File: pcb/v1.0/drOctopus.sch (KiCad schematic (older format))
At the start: 47 parts, among them CON1 Servo, CON2 Servo, CON3 Heater, CON4 +12V, CON5 BEC, CON6 Motor, CON7 FAN1, CON8 FAN2, Q1 16MHz, SW1 RESET, T1 IRLR2905PBF, T2 IRLML6244TRPBF, T3 IRLML6244TRPBF, T4 IRLML6244TRPBF, U1 ATmega328-AU, U2 78M05CDT, U3 ESP-01, U4 AMS1117-3.3

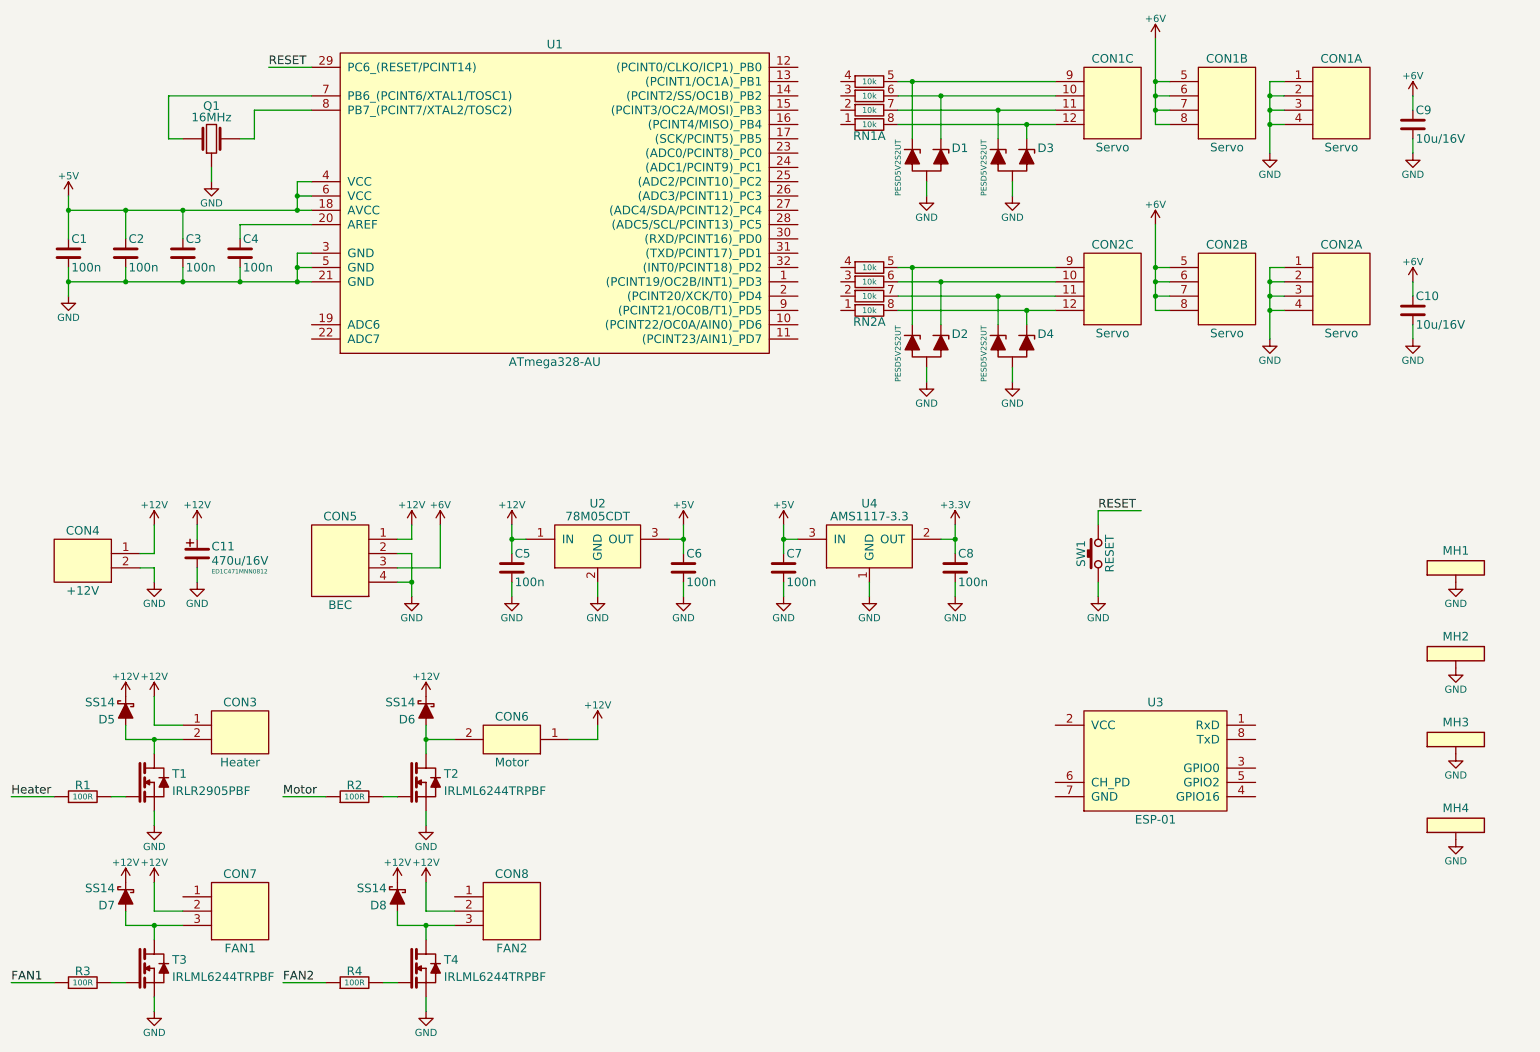
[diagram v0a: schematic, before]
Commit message: Working on new PCB
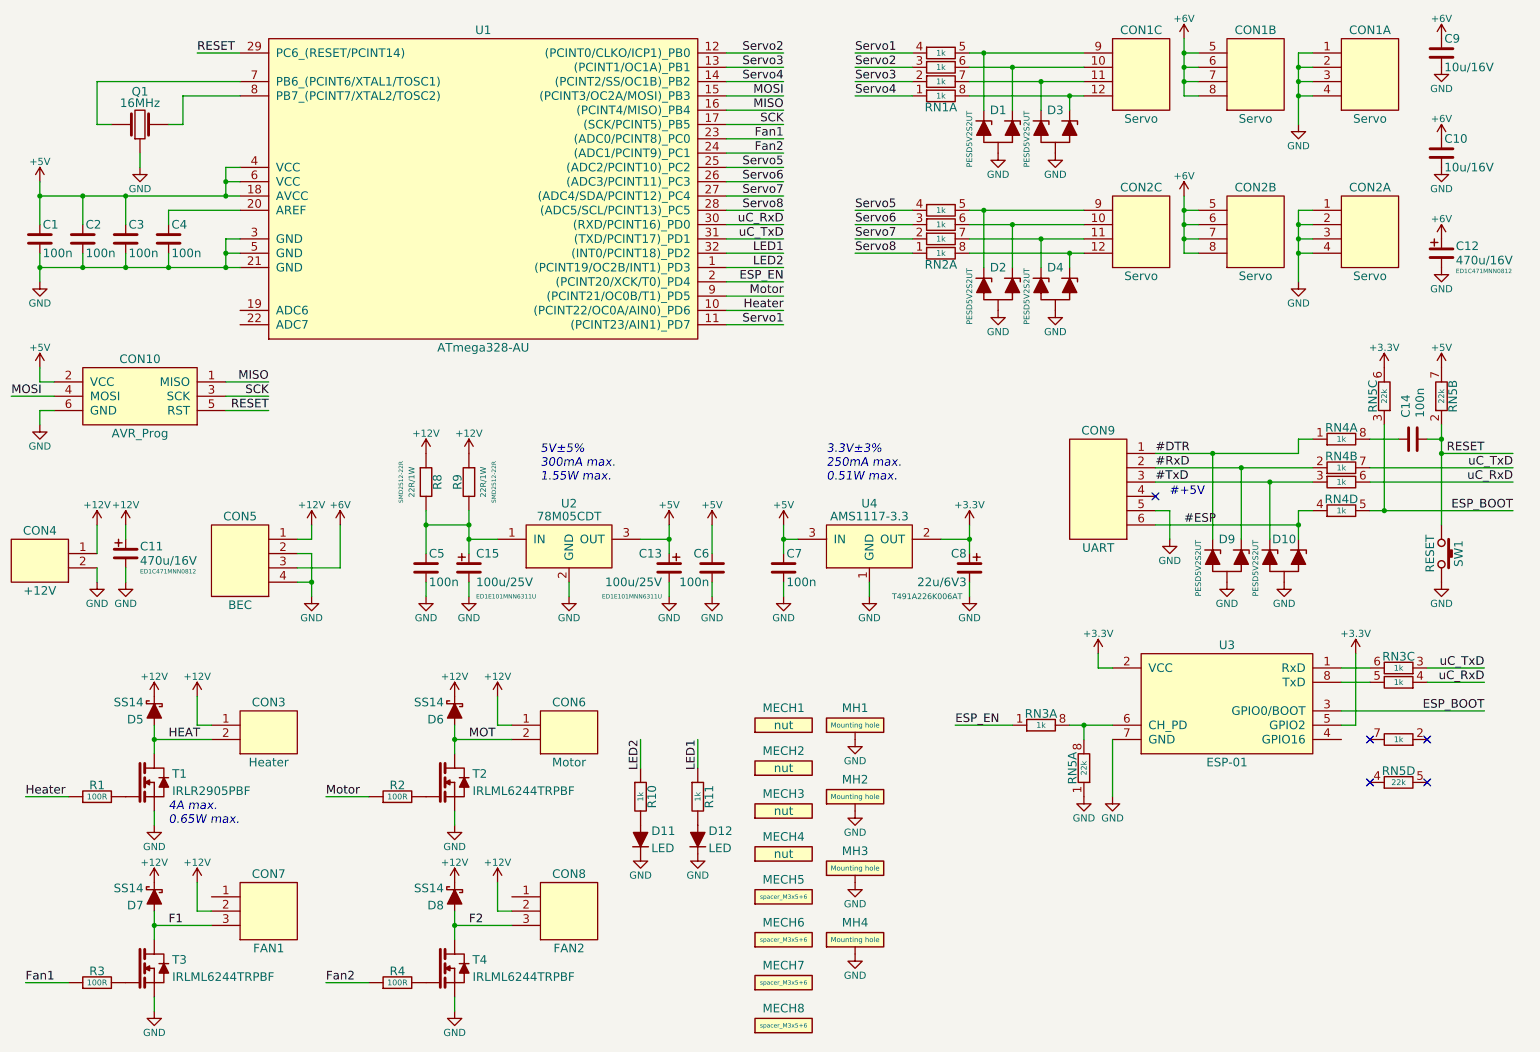
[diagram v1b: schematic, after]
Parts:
- removed C8: 100n, 0603_N, symbol C
- removed CON6: Motor, PIN-2x1_angled_N, symbol PIN-2x1_angled
- removed U3: ESP-01, ESP-01_N_socket, symbol ESP-01-RESCUE-drOctopus
- added C12: 470u/16V, Cpol_8.0_12.0_M, symbol Cpol
- added C13, C15: 100u/25V, Cpol_6.3_11.0_N, symbol Cpol
- added C14: 100n, 0603_N, symbol C
- added C8: 22u/6V3, Tantal_A_N, symbol Cpol
- added CON10: AVR_Prog, PIN-2x3_N, symbol AVR_Prog
- added CON6: Motor, PIN-2x1_angled_N, symbol PIN-1x2
- added CON9: UART, PIN-1x6_angled_N, symbol PIN-1x6_angled
- added D10, D9: PESD5V2S2UT, SOT23-3_N, symbol PESD5V2S2UT
- added D11, D12: LED, 0805_N, symbol diode
- added MECH1, MECH2, MECH3, MECH4: nut, nut_M3_DIN985, symbol nut_M3_DIN985
- added MECH5, MECH6, MECH7, MECH8: spacer_M3x5+6, spacer_M3x5+6, symbol spacer_M3x5+6
- added R10, R11: 1k, 0603_N, symbol R
- added R8, R9: 22R/1W, 2512_N, symbol R
- added RN3, RN4: 1k, 4x0603_N, symbol R_Network_4
- added RN5: 22k, 4x0603_N, symbol R_Network_4
- added U3: ESP-01, ESP-01_N_socket, symbol ESP-01
- MH1, MH2, MH3, MH4: value mounting_hole_plated -> Mounting hole
- RN1, RN2: value 10k -> 1k
- T1, U2: footprint D-PAK_M -> D-PAK_N
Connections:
- net FAN1 is gone; now on net Fan1: R3.1
- net FAN2 is gone; now on net Fan2: R4.1
- net +12V: now also CON6.1, R8.1, R9.1; no longer C5.1, U2.1 (IN)
- net +3V3: now also C8.1, RN5.6 (2), U3.2 (VCC), U3.5 (GPIO2)
- net +5V: now also C13.1, CON10.2 (VCC), RN5.7 (2)
- net +6V: now also C12.1
- net GND: now also C12.2, C13.2, C15.2, C8.2, CON10.6 (GND), CON9.5, D10.3 (A), D11.1 (A), D12.1 (A), D9.3 (A), RN5.1, U3.7 (GND)
- net Heater: now also U1.10 ((PCINT22/OC0A/AIN0)_PD6)
- net Motor: now also U1.9 ((PCINT21/OC0B/T1)_PD5)
- net RESET: now also C14.2, CON10.5 (RST), RN5.2 (1)
- net LED2: now reaches U1.1 ((PCINT19/OC2B/INT1)_PD3)
- net LED2: now also R10.1
- net Servo1: now reaches U1.11 ((PCINT23/AIN1)_PD7)
- net Servo1: now also RN1.4 (1)
- net Servo2: now reaches U1.12 ((PCINT0/CLKO/ICP1)_PB0)
- net Servo2: now also RN1.3 (1)
- net Servo3: now reaches U1.13 ((PCINT1/OC1A)_PB1)
- net Servo3: now also RN1.2 (1)
- net Servo4: now reaches U1.14 ((PCINT2/SS/OC1B)_PB2)
- net Servo4: now also RN1.1
- net MOSI: now reaches U1.15 ((PCINT3/OC2A/MOSI)_PB3)
- net MOSI: now also CON10.4 (MOSI)
- net MISO: now reaches U1.16 ((PCINT4/MISO)_PB4)
- net MISO: now also CON10.1 (MISO)
- net SCK: now reaches U1.17 ((SCK/PCINT5)_PB5)
- net SCK: now also CON10.3 (SCK)
- net ESP_EN: now reaches U1.2 ((PCINT20/XCK/T0)_PD4)
- net ESP_EN: now also RN3.1
- net Fan1: now reaches U1.23 ((ADC0/PCINT8)_PC0)
- net Fan2: now reaches U1.24 ((ADC1/PCINT9)_PC1)
- net Servo5: now reaches U1.25 ((ADC2/PCINT10)_PC2)
- net Servo5: now also RN2.4 (1)
- net Servo6: now reaches U1.26 ((ADC3/PCINT11)_PC3)
- net Servo6: now also RN2.3 (1)
- net Servo7: now reaches U1.27 ((ADC4/SDA/PCINT12)_PC4)
- net Servo7: now also RN2.2 (1)
- net Servo8: now reaches U1.28 ((ADC5/SCL/PCINT13)_PC5)
- net Servo8: now also RN2.1
- net uC_RxD: now reaches U1.30 ((RXD/PCINT16)_PD0)
- net uC_RxD: now also RN3.4 (1), RN4.6 (2)
- net uC_TxD: now reaches U1.31 ((TXD/PCINT17)_PD1)
- net uC_TxD: now also RN3.3 (1), RN4.7 (2)
- net LED1: now reaches U1.32 ((INT0/PCINT18)_PD2)
- net LED1: now also R11.1
- net HEAT: now reaches CON3.2, D5.2 (C), T1.2 (D)
- net MOT: now reaches D6.2 (C), T2.3 (D)
- net MOT: now also CON6.2
- net F1: now reaches CON7.3, D7.2 (C), T3.3 (D)
- net F2: now reaches CON8.3, D8.2 (C), T4.3 (D)
- new net: C15.1, C5.1, R8.2, R9.2, U2.1 (IN)
- new net: RN3.8 (2), RN5.8 (2), U3.6 (CH_PD)
- new net: RN3.5 (2), U3.8 (TxD)
- new net: RN3.6 (2), U3.1 (RxD)
- new net: C14.1, RN4.8 (2)
- new net: D11.2 (C), R10.2
- new net: D12.2 (C), R11.2
- new net #DTR: CON9.1, D9.1 (C1), RN4.1
- new net #ESP: CON9.6, D10.2 (C2), RN4.4 (1)
- new net #RxD: CON9.2, D9.2 (C2), RN4.2 (1)
- new net #TxD: CON9.3, D10.1 (C1), RN4.3 (1)
- new net ESP_BOOT: RN4.5 (2), RN5.3 (1), U3.3 (GPIO0/BOOT)
- no-connect marks 0 -> 5
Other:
- note added: "#+5V"
- note added: "3.3V±3%\n250mA max.\n0.51W max."
- note added: "4A max.\n0.65W max."
- note added: "5V±5%\n300mA max.\n1.55W max."
- moved on the sheet: C1, C10, C11, C2, C3, C4, C5, C6, C9, CON1A, CON1B, CON1C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
